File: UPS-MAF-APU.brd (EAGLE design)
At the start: 65 x 56 mm, 32 parts, among them J1 CONNECTOR_PI_40_PIN, J2 Barrel DC In, J3 OLED, J4 OSTOQ045451, J5 External DS18B20 Temp, J6 FTDI Serial Console, J7 MagJack, U1 OLED_I2C, U2 SI7006-A20-IM, U4 INA260AIPW, U6 ENC28J60_SS, U7 5V SMPS, Y1 ECS-250-20-3X-EN-TR

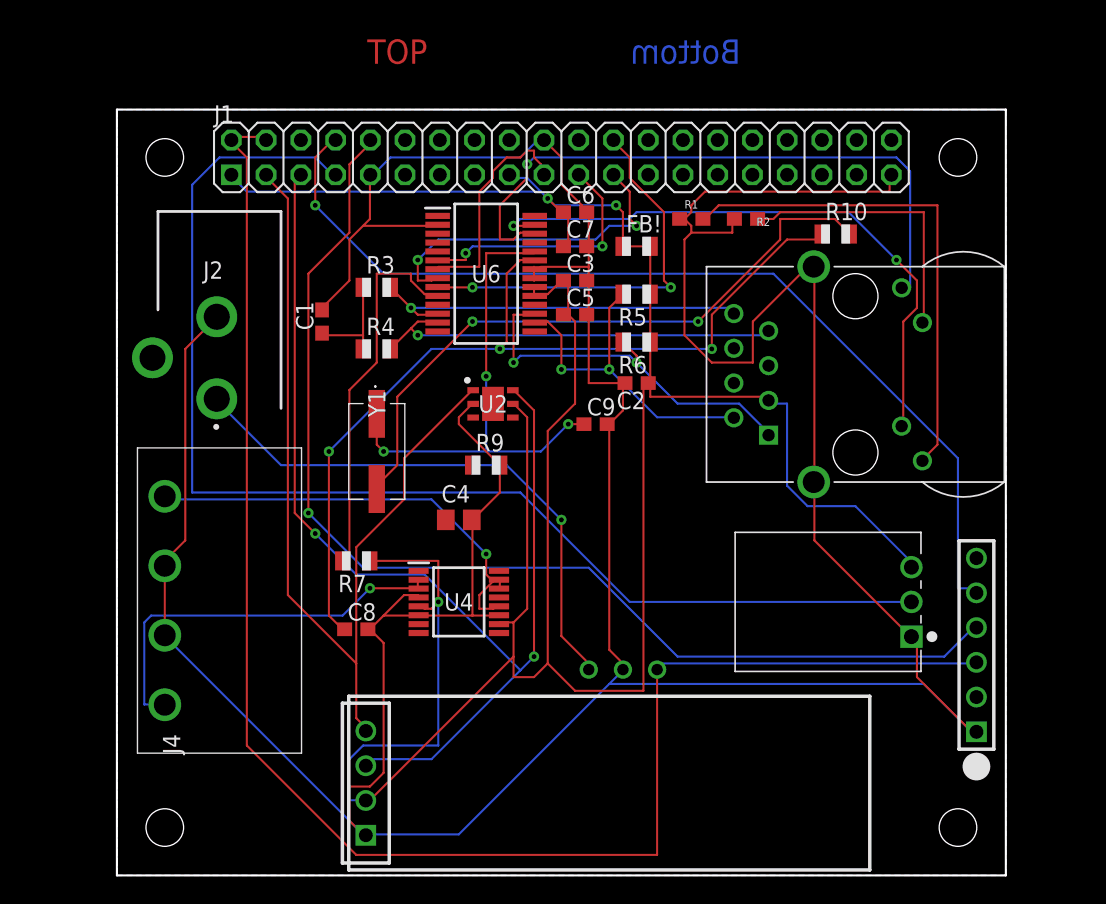
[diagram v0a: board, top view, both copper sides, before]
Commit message: README
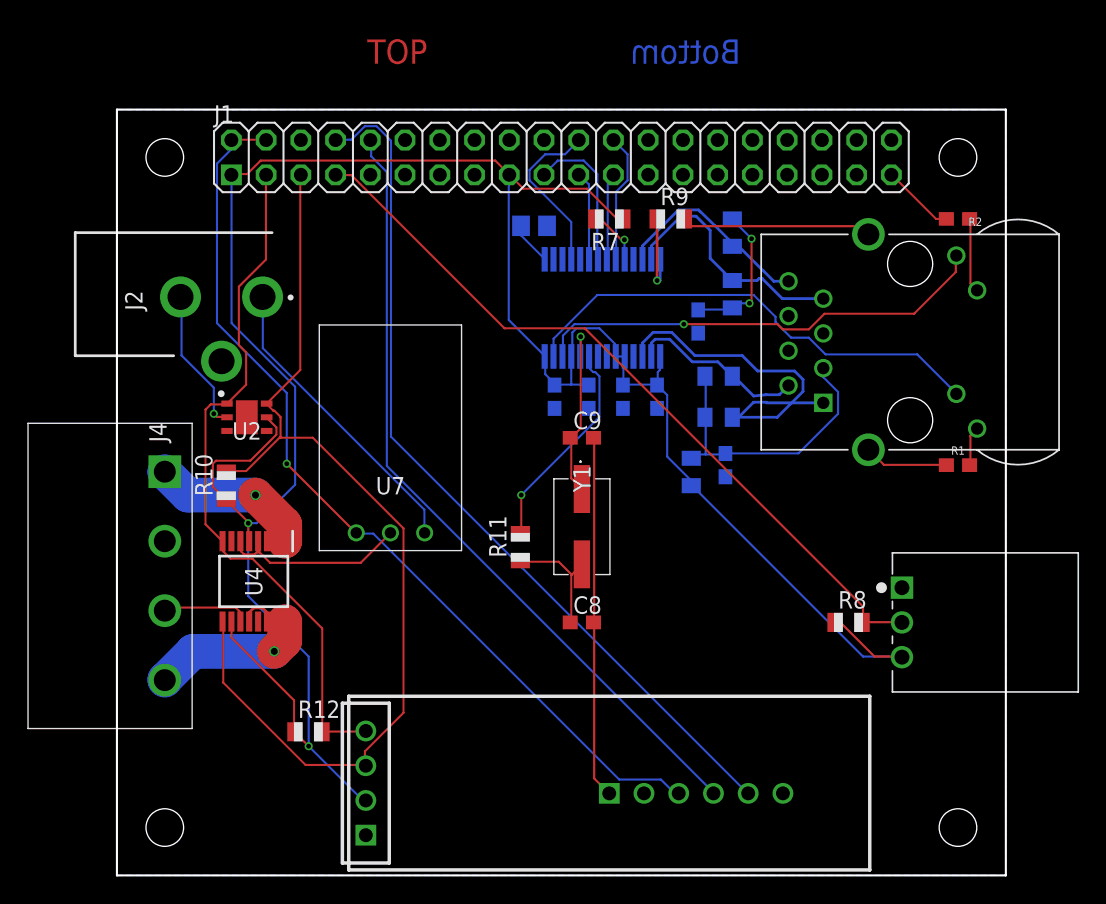
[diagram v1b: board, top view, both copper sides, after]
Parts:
- removed FB!: 600 uH, adafruit:R0805
- added FB1: 600 uH, adafruit:R0805
- added R11: 0, adafruit:R0805
- added R12, R8: 4.7K, adafruit:R0805
- C9: value 100nF -> 18pF
- R10: value 0 -> 4.7K
- moved R10 48.2 mm to (8.00, 28.5), turned to 90 degrees
- moved R7 31.1 mm to (36.0, 48.0)
- moved C1 27.5 mm to (42.5, 40.5), flipped to the bottom, turned to 270 degrees
- moved J6 27.2 mm to (36.0, 6.00), flipped to the bottom, turned to 180 degrees
- moved R1 26.5 mm to (61.5, 30.0)
- moved R3 26.3 mm to (45.0, 47.0), flipped to the bottom, turned to 270 degrees
- moved R4 26.3 mm to (45.0, 42.5), flipped to the bottom, turned to 90 degrees
- moved R9 22.5 mm to (40.5, 48.0)
- moved C4 22.2 mm to (30.5, 47.5), flipped to the bottom, turned to 180 degrees
- moved U7 19.7 mm to (20.0, 32.0), flipped to the top
- moved U2 18.0 mm to (9.50, 33.5)
- moved J4 17.0 mm to (3.50, 29.5), turned to 270 degrees
- moved C8 16.5 mm to (34.0, 18.5)
- moved Y1 16.0 mm to (34.0, 25.5)
- moved R2 15.5 mm to (61.5, 48.0)
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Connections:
- net TPIN+ renamed TPIN_P
- net TPIN- renamed TPIN_N
- net TPOUT+ renamed TPOUT_P
- net TPOUT- renamed TPOUT_N
- new net N$1: C2.1, FB1.2, J7.R3, R5.1, R6.1
- net 3.3V: now also FB1.1, R10.1, R12.1, R8.1; no longer C2.1, FB!.1, FB!.2, J7.R3, R5.1, R6.1
- net N$2: now also C8.1, R11.1; no longer R10.2
- net N$4: now also R8.2
- net OOUT: now also R11.2; no longer C8.1, R10.1
- net SCK: now also R10.2
- net SDA: now also R12.2
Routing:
- net GND: track 312.3 -> 83.0 mm, vias 0 -> 1
- net 5V: track 118.1 -> 67.5 mm, vias 0 -> 1
- net OOUT: track 66.0 -> 15.8 mm, vias 3 -> 1
- net N$2: track 47.2 -> 8.81 mm, vias 2 -> 0
- net 3.3V: track 216.0 -> 179.7 mm, vias 3 -> 2
- net N$4: track 90.2 -> 55.7 mm
- net N$7: track 36.7 -> 2.91 mm
- net RX_OT: track 83.2 -> 58.2 mm, vias 1 -> 0
- net OIN: track 36.6 -> 13.3 mm, vias 3 -> 1
- net RST: track 27.4 -> 4.18 mm, vias 0 -> 1
- net N$1: track 0.00 -> 21.7 mm
- net CS: track 29.5 -> 9.50 mm, vias 2 -> 0
- net VIN: track 40.7 -> 22.2 mm, vias 1 -> 0
- net BATTERY+: track 32.6 -> 14.3 mm
- net SCLK: track 24.4 -> 6.39 mm, vias 2 -> 0
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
